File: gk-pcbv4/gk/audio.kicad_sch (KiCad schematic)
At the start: 21 parts, among them J12 AudioJack3_SwitchTR, J13 Conn_01x02, U16 TAD5112, U17 PAM8302AAS

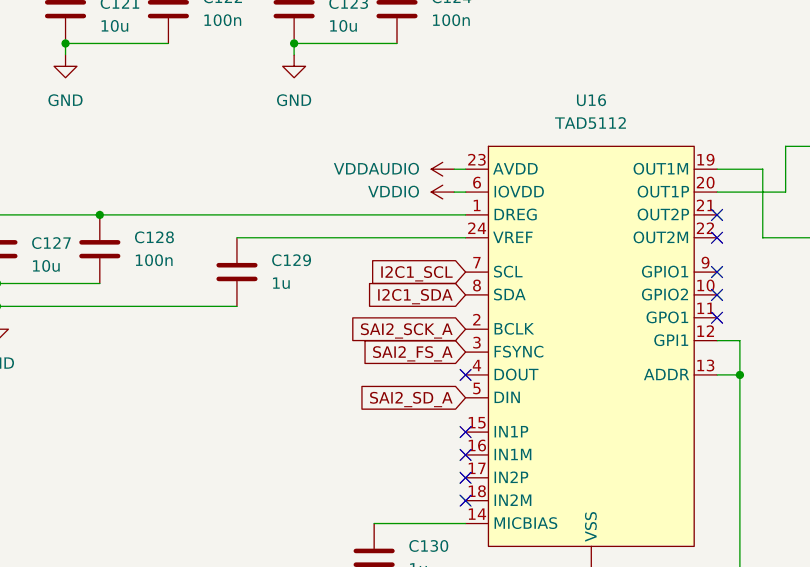
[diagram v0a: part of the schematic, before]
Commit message: pcb order 20251115
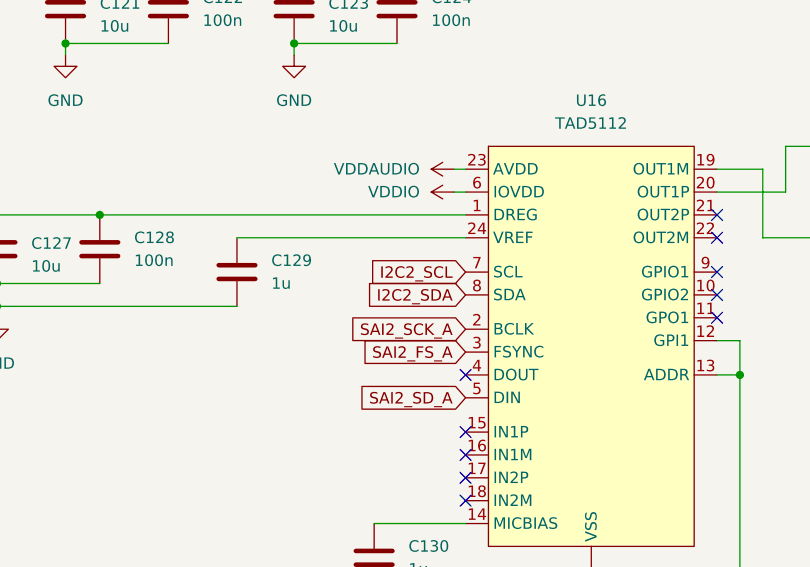
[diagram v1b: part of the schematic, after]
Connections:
- net I2C1_SCL renamed I2C2_SCL
- net I2C1_SDA renamed I2C2_SDA
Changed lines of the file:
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@@
 		)
 	)
-	(global_label "I2C1_SCL"
+	(global_label "I2C2_SCL"
 		(shape input)
 		(at 76.2 59.69 180)
@@
 		)
 	)
-	(global_label "I2C1_SDA"
+	(global_label "I2C2_SDA"
 		(shape input)
 		(at 76.2 62.23 180)
